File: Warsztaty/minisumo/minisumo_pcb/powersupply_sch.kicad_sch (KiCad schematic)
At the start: 8 parts, among them J2 Conn_01x02_Pin, Q1 PMOS, U7 LM1117S-5.0, U9 LM1117S-3.3

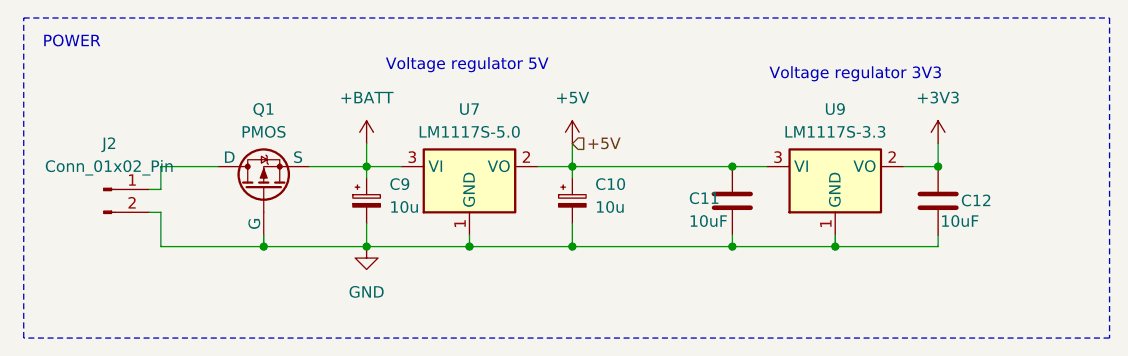
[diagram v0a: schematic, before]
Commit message: chyba gotowy schemat
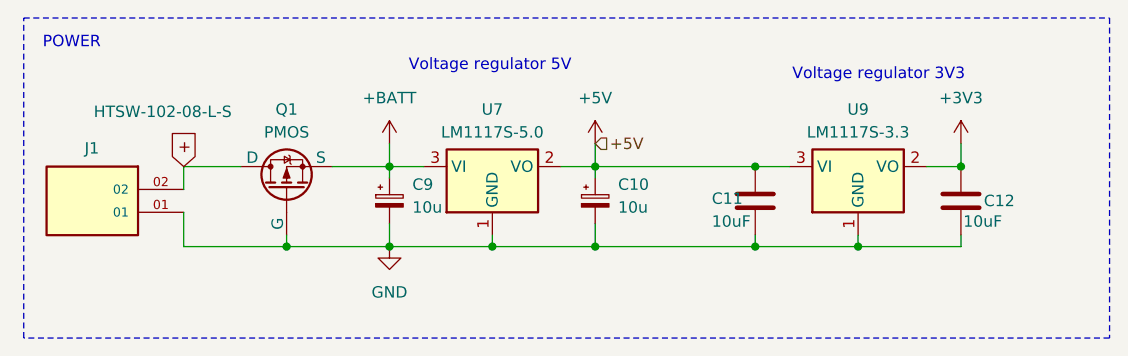
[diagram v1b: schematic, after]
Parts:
- removed J2: Conn_01x02_Pin, symbol Connector:Conn_01x02_Pin
- added J1: HTSW-102-08-L-S, HTSW-102-08-L-S:SAMTEC_HTSW-102-08-L-S, symbol HTSW-102-08-L-S:HTSW-102-08-L-S
- C10, C11, C12, C9: footprint (none) -> Capacitor_SMD:C_0805_2012Metric_Pad1.18x1.45mm_HandSolder
- Q1: footprint (none) -> Package_TO_SOT_SMD:SOT-23-3
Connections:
- net GND: now also J1.01
- net +: now reaches Q1.1 (D)
- net +: now also J1.02
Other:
- moved on the sheet: C10, C11, C12, C9, Q1, U7, U9

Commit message: chyba gotowy schemat
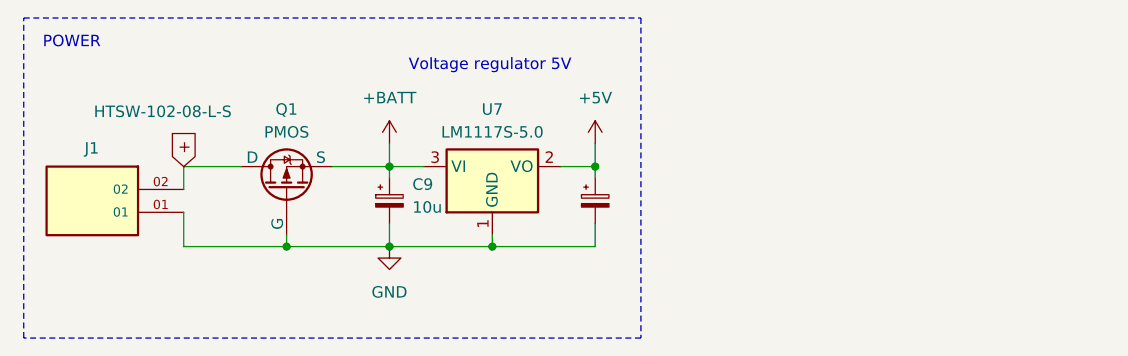
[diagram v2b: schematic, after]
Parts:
- removed C11, C12: 10uF, Capacitor_SMD:C_0805_2012Metric_Pad1.18x1.45mm_HandSolder, symbol Device:C
- removed U9: LM1117S-3.3, Package_TO_SOT_SMD:TO-263-3_TabPin2, symbol Regulator_Linear:LM1117S-3.3
- C10, C9: footprint Capacitor_SMD:C_0805_2012Metric_Pad1.18x1.45mm_HandSolder -> Capacitor_Tantalum_SMD:CP_EIA-3528-12_Kemet-T
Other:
- note removed: "Voltage regulator 3V3"

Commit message: stan przed usunięciem jednego czujnika lini
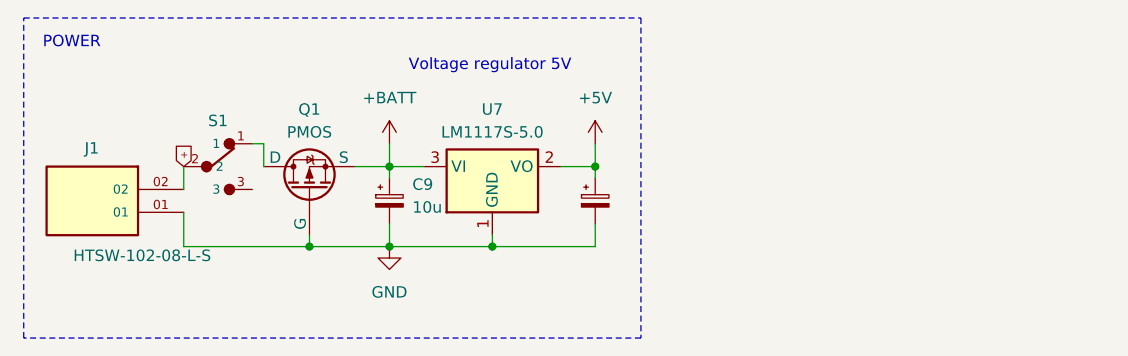
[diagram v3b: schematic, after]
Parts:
- added S1: 1101M2S3CQE2, 1101M2S3CQE2:SW_1101M2S3CQE2, symbol 1101M2S3CQE2:1101M2S3CQE2
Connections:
- net +: now also S1.2; no longer Q1.1 (D)
- new net: Q1.1 (D), S1.1
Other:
- moved on the sheet: Q1
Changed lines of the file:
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@@
 	)
 	(junction
-		(at 43.18 40.64)
+		(at 45.72 40.64)
 		(diameter 0)
 		(color 0 0 0 0)
@@
 	(wire
 		(pts
-			(xy 43.18 39.37) (xy 43.18 40.64)
-		)
-		(stroke
-			(width 0)
-			(type default)
-		)
-	)
-	(wire
-		(pts
-			(xy 43.18 40.64) (xy 31.75 40.64)
+			(xy 45.72 39.37) (xy 45.72 40.64)
+		)
+		(stroke
+			(width 0)
+			(type default)
+		)
+	)
+	(wire
+		(pts
+			(xy 31.75 40.64) (xy 45.72 40.64)
 		)
 		(stroke
@@
 	(wire
 		(pts
-			(xy 31.75 31.75) (xy 38.1 31.75)
+			(xy 40.64 29.21) (xy 40.64 31.75)
+		)
+		(stroke
+			(width 0)
+			(type default)
+		)
+	)
+	(wire
+		(pts
+			(xy 45.72 40.64) (xy 54.61 40.64)
 		)
 		(stroke
@@
 	(wire
 		(pts
-			(xy 48.26 31.75) (xy 54.61 31.75)
-		)
-		(stroke
-			(width 0)
-			(type default)
-		)
-	)
-	(wire
-		(pts
-			(xy 43.18 40.64) (xy 54.61 40.64)
+			(xy 50.8 31.75) (xy 54.61 31.75)
 		)
 		(stroke
@@
 		(pts
 			(xy 73.66 31.75) (xy 77.47 31.75)
+		)
+		(stroke
+			(width 0)
+			(type default)
+		)
+	)
+	(wire
+		(pts
+			(xy 39.37 29.21) (xy 40.64 29.21)
 		)
 		(stroke
@@
 		(effects
 			(font
-				(size 1.27 1.27)
+				(size 0.762 0.762)
 			)
 			(justify left)
 		)
 		(property "Intersheetrefs" "${INTERSHEET_REFS}"
-			(at 31.75 27.1924 90)
+			(at 31.75 29.0152 90)
 			(effects
 				(font
@@
 		)
 		(property "Value" "HTSW-102-08-L-S"
-			(at 37.084 25.654 0)
+			(at 34.798 41.656 0)
 			(effects
 				(font
@@
 	(symbol
 		(lib_id "Simulation_SPICE:PMOS")
-		(at 43.18 34.29 90)
+		(at 45.72 34.29 90)
 		(unit 1)
 		(exclude_from_sim no)
@@
 		(fields_autoplaced yes)
 		(property "Reference" "Q1"
-			(at 43.18 25.4 90)
+			(at 45.72 25.4 90)
 			(effects
 				(font
@@
 		)
 		(property "Value" "PMOS"
-			(at 43.18 27.94 90)
+			(at 45.72 27.94 90)
 			(effects
 				(font
@@
 		)
 		(property "Footprint" "Package_TO_SOT_SMD:SOT-23-3"
-			(at 40.64 29.21 0)
+			(at 43.18 29.21 0)
 			(effects
 				(font
@@
 		)
 		(property "Datasheet" "https://ngspice.sourceforge.io/docs/ngspice-html-manual/manual.xhtml#cha_MOSFETs"
-			(at 55.88 34.29 0)
+			(at 58.42 34.29 0)
 			(effects
 				(font
@@
 		)
 		(property "Description" "P-MOSFET transistor, drain/source/gate"
-			(at 43.18 34.29 0)
+			(at 45.72 34.29 0)
 			(effects
 				(font
@@
 		)
 		(property "Sim.Device" "PMOS"
-			(at 60.325 34.29 0)
+			(at 62.865 34.29 0)
 			(effects
 				(font
@@
 		)
 		(property "Sim.Type" "VDMOS"
-			(at 62.23 34.29 0)
+			(at 64.77 34.29 0)
 			(effects
 				(font
@@
 		)
 		(property "Sim.Pins" "1=D 2=G 3=S"
-			(at 58.42 34.29 0)
+			(at 60.96 34.29 0)
 			(effects
 				(font
@@
 					(unit 1)
 				)
+			)
+		)
+	)
+	(symbol
+		(lib_id "1101M2S3CQE2:1101M2S3CQE2")
+		(at 34.29 31.75 0)
+		(unit 1)
+		(exclude_from_sim no)
+		(in_bom yes)
+		(on_board yes)
+		(dnp no)
+		(fields_autoplaced yes)
+		(property "Reference" "S1"
+			(at 35.56 26.67 0)
+			(effects
+				(font
+					(size 1.27 1.27)
+				)
+			)
+		)
+		(property "Value" "1101M2S3CQE2"
+			(at 35.56 26.67 0)
+			(effects
+				(font
+					(size 1.27 1.27)
+				)
+				(hide yes)
+			)
+		)
+		(property "Footprint" "1101M2S3CQE2:SW_1101M2S3CQE2"
+			(at 34.29 31.75 0)
+			(effects
+				(font
+					(size 1.27 1.27)
+				)
+				(justify bottom)
+				(hide yes)
+			)
+		)
+		(property "Datasheet" ""
+			(at 34.29 31.75 0)
+			(effects
+				(font
+					(size 1.27 1.27)
+				)
+				(hide yes)
+			)
+		)
+		(property "Description" ""
+			(at 34.29 31.75 0)
+			(effects
+				(font
+					(size 1.27 1.27)
+				)
+				(hide yes)
+			)
+		)
+		(property "MF" "C&K"
+			(at 34.29 31.75 0)
+			(effects
+				(font
+					(size 1.27 1.27)
+				)
+				(justify bottom)
+				(hide yes)
+			)
+		)
+		(property "Description_1" "\nSlide Switch SPDT Through Hole\n"
+			(at 34.29 31.75 0)
+			(effects
+				(font
+					(size 1.27 1.27)
+				)
+				(justify bottom)
+				(hide yes)
+			)
+		)
+		(property "Package" "None"
+			(at 34.29 31.75 0)
+			(effects
+				(font
+					(size 1.27 1.27)
+				)
+				(justify bottom)
+				(hide yes)
+			)
+		)
+		(property "Price" "None"
+			(at 34.29 31.75 0)
+			(effects
+				(font
+					(size 1.27 1.27)
+				)
+				(justify bottom)
+				(hide yes)
+			)
+		)
+		(property "Check_prices" "https://www.snapeda.com/parts/1101-M2S3CQE2/C%2526K/view-part/?ref=eda"
+			(at 34.29 31.75 0)
+			(effects
+				(font
+					(size 1.27 1.27)
+				)
+				(justify bottom)
+				(hide yes)
+			)
+		)
+		(property "SnapEDA_Link" "https://www.snapeda.com/parts/1101-M2S3CQE2/C%2526K/view-part/?ref=snap"
+			(at 34.29 31.75 0)
+			(effects
+				(font
+					(size 1.27 1.27)
+				)
+				(justify bottom)
+				(hide yes)
+			)
+		)
+		(property "MP" "1101-M2S3CQE2"
+			(at 34.29 31.75 0)
+			(effects
+				(font
+					(size 1.27 1.27)
+				)
+				(justify bottom)
+				(hide yes)
+			)
+		)
+		(property "Availability" "In Stock"
+			(at 34.29 31.75 0)
+			(effects
+				(font
+					(size 1.27 1.27)
+				)
+				(justify bottom)
+				(hide yes)
+			)
+		)
+		(property "MANUFACTURER" "CnK"
+			(at 34.29 31.75 0)
+			(effects
+				(font
+					(size 1.27 1.27)
+				)
+				(justify bottom)
+				(hide yes)
+			)
+		)
+		(pin "3"
+		)
+		(pin "2"
+		)
+		(pin "1"
+		)
+		(instances
+			(project "minisumo_pcb"
+				(path "/7b99a4ad-c15f-48f5-acdf-b2b295c8ee3b/fec592cb-397f-40c8-9127-e83f29739826"
+					(reference "S1")
+					(unit 1)
+				)
